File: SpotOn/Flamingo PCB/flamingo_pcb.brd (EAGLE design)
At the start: 86 x 131 mm, 32 parts, among them J1 1725698, J2 ADAFRUIT_1X2-3.5MM, J3 1725672, J5 PTH, J8 PTH

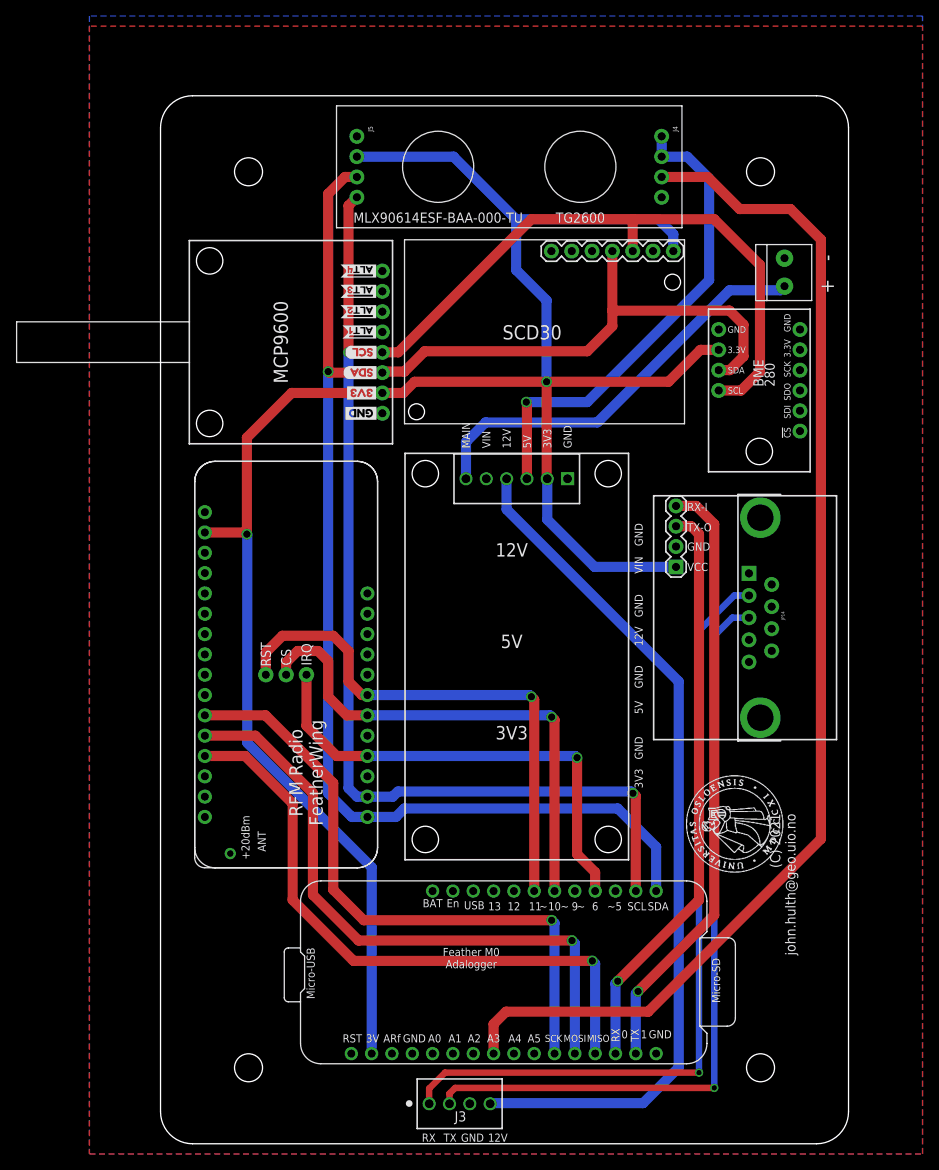
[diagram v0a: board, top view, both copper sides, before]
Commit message: Flamingo PCB radio
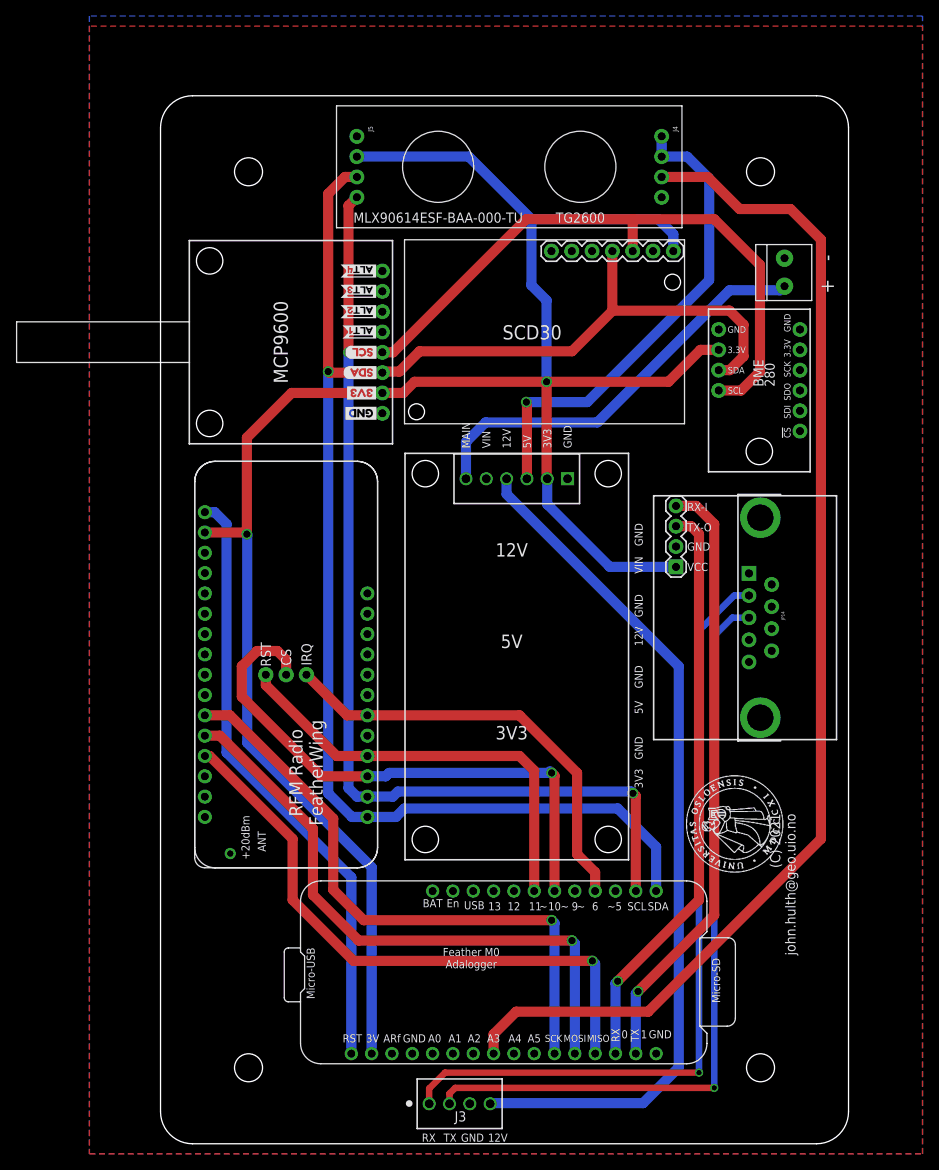
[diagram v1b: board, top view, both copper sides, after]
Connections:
- removed net N$25: MS2.1
- net !RESET: now also MS2.1
- net CS: now also MS2.19; no longer MS2.22
- net E: now also MS2.23; no longer MS2.19
- net IRQ: now also MS2.22; no longer MS2.20
- net RST: now also MS2.20; no longer MS2.23
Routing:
- net !RESET: track 0.00 -> 76.0 mm
- net RST: track 66.7 -> 54.3 mm, vias 1 -> 0
- net CS: track 63.2 -> 70.7 mm
- net IRQ: track 59.5 -> 54.6 mm, vias 1 -> 0
- net MOSI: track 78.2 -> 75.6 mm
- net MISO: track 77.8 -> 75.2 mm
- net SCK: track 78.6 -> 76.0 mm
- net 3V3: track 255.7 -> 253.8 mm
- net SDA: track 201.8 -> 200.7 mm
- net A3: track 152.3 -> 151.5 mm
